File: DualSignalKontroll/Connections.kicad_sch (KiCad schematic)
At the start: 15 parts, among them J10 Power Out, J11 Buttons and switches, J12 Buttons and switches, J13 Power Out, J14 Buttons and switches, SW2 Switch A, SW3 Switch B, SW4 Select A, SW5 Select B, SW6 Switch A, SW7 Switch B

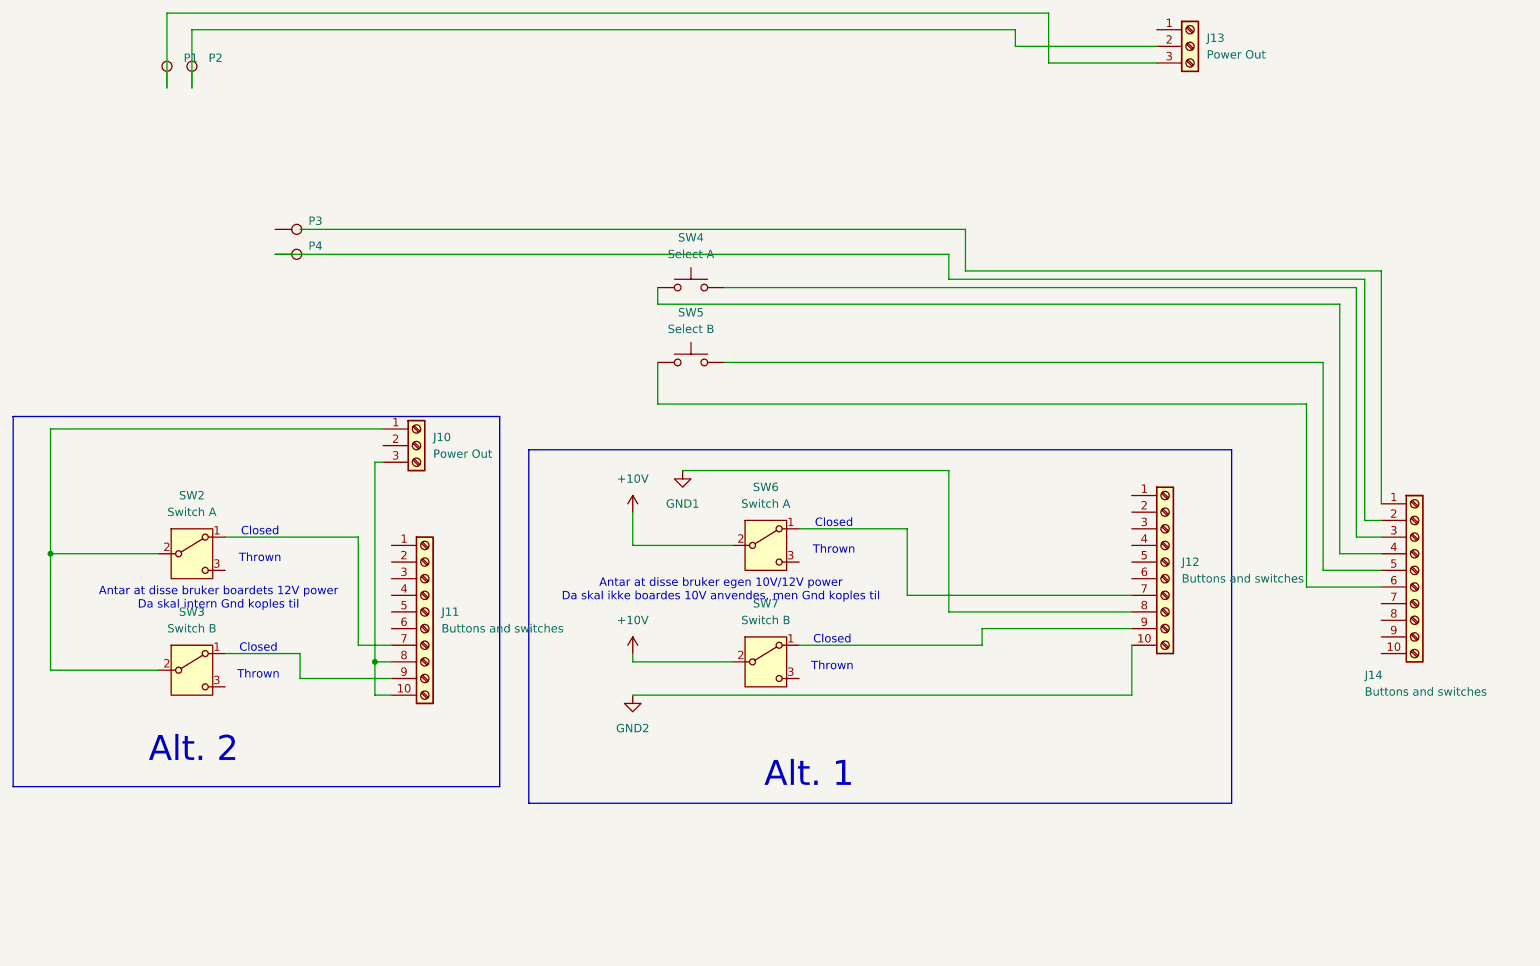
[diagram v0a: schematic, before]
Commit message: Started on V2
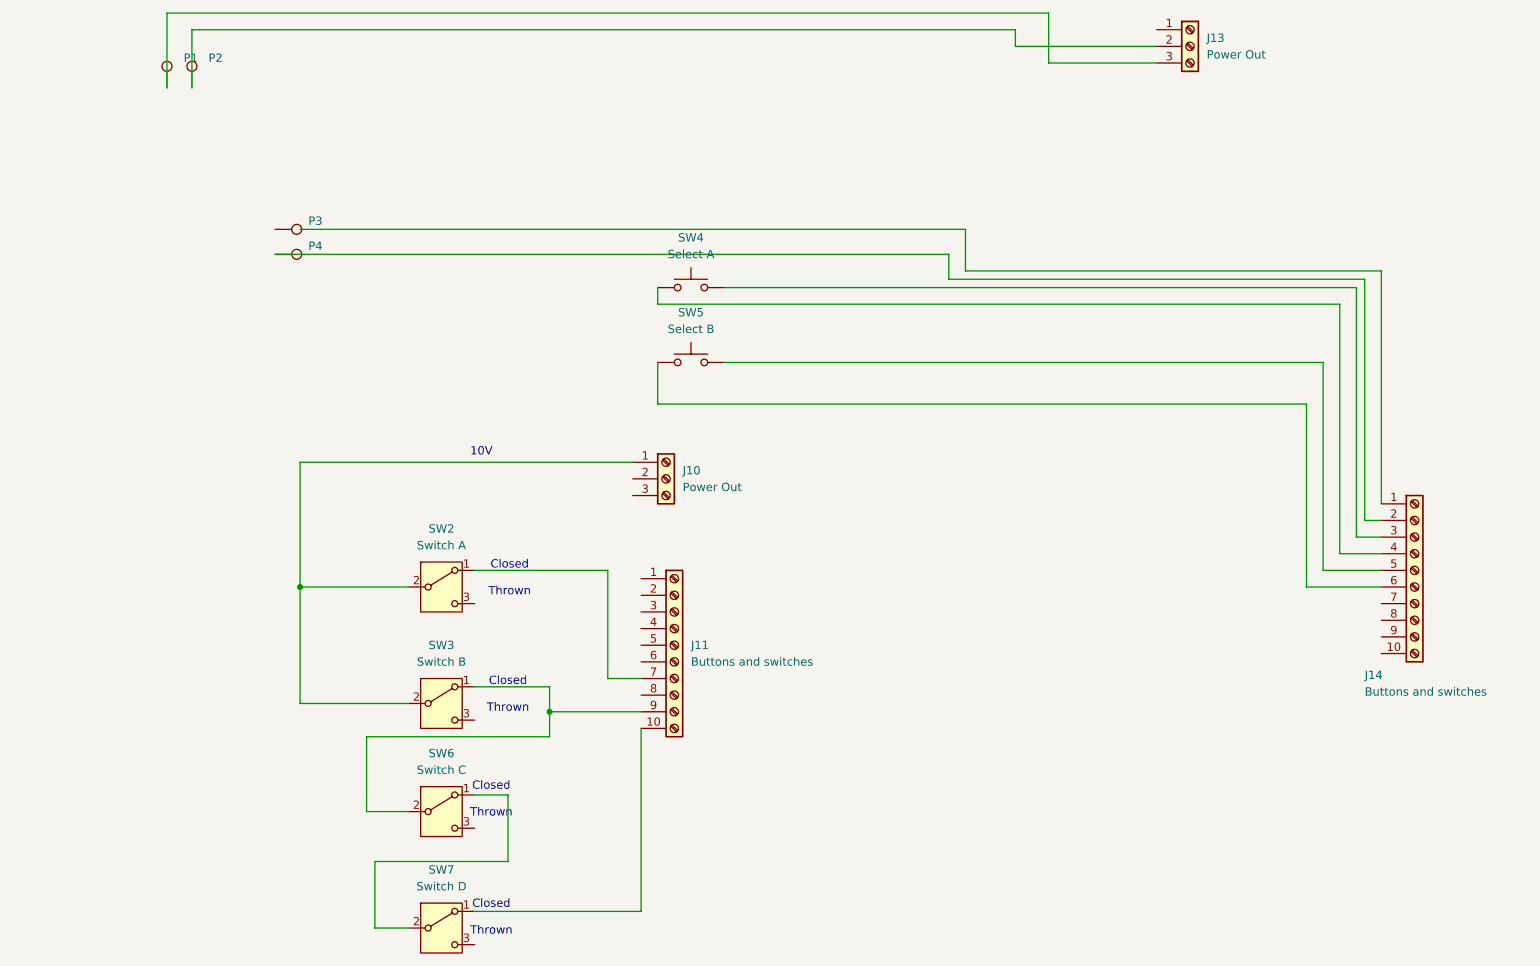
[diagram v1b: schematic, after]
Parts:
- removed J12: Buttons and switches, symbol Connector:Screw_Terminal_01x10
- SW6: value Switch A -> Switch C
- SW7: value Switch B -> Switch D
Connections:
- net at SW6.1 (A): now also SW7.2 (B)
- net at SW7.1 (A): now also J11.10 (Pin_10)
- net at J11.9 (Pin_9), SW3.1 (A): now also SW6.2 (B)
- removed net +10V: SW6.2 (B), SW7.2 (B)
- now unconnected: J10.3 (Pin_3), J11.8 (Pin_8)
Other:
- note added: "10V"
- note removed: "Alt. 1"
- note removed: "Alt. 2"
- note removed: "Antar at disse bruker boardets 12V power Da skal intern Gnd koples til"
- note removed: "Antar at disse bruker egen 10V/12V power Da skal ikke boardes 10V anvendes, men Gnd koples til"
- moved on the sheet: J10, J11, SW2, SW3
